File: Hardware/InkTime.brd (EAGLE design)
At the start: 46 x 35 mm, 105 parts, among them IC1 BQ25180YBGR, IC2 DRV2605YZFR, IC3 BMA423, IC9 RT6160AWSC, J1 503480-2400, J2 TC2030-IDC, J4 KH-TYPE-C-16P, Q1 20V/4.2A/52mΩ/1.4W, Q3 SI1308EDL-T1-GE3, U1 NRF52840_QF, U3 MAX17048G+T10, X1 32MHz, X2 32.768kHz

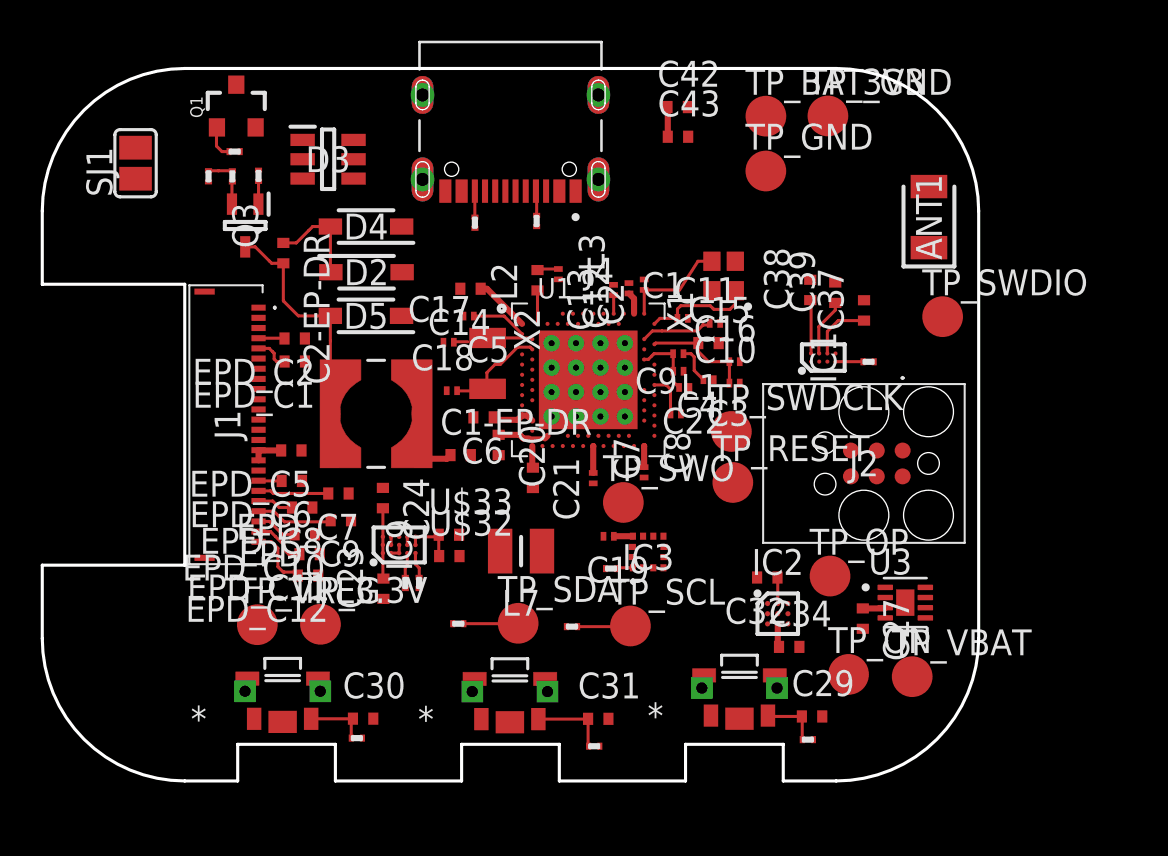
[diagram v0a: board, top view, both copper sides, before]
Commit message: Add files via upload
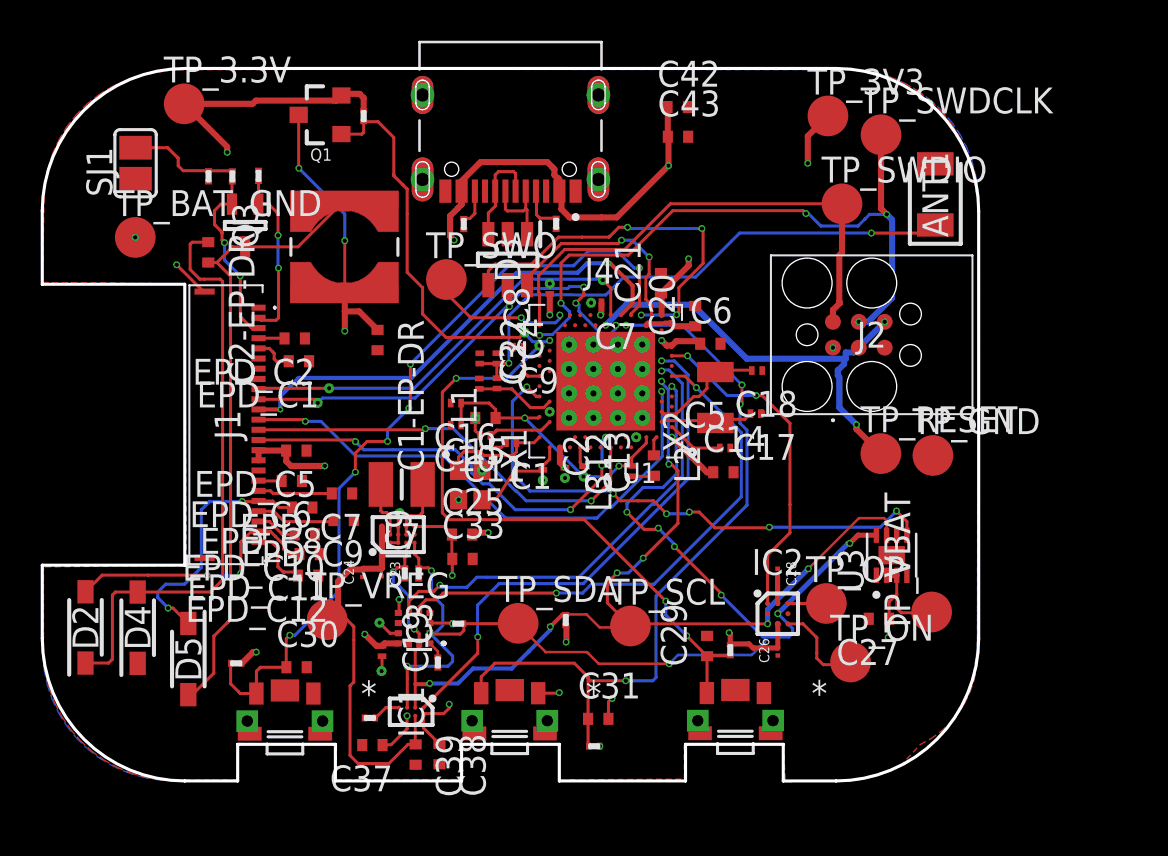
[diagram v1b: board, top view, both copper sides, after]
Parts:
- removed C32: 1uF, InkTime_v5:NORDIC_NRF_3_RESC0402_L
- removed C34: 0.1uF, InkTime_v5:NORDIC_NRF_3_RESC0402_L
- removed U$32, U$33: (no value), InkTime_v5:NORDIC_NRF_3_RESC0402_L
- added C25, C33: (no value), InkTime_v5:NORDIC_NRF_3_RESC0402_L
- added C26, C28: 0.1uF, InkTime_v5:GRM011R60J152KE01L_2_CAPC0201X13N
- C23, C24: device InkTime_v5:NORDIC_NRF_3_RESC0402_L -> InkTime_v5:GRM011R60J152KE01L_2_CAPC0201X13N
- moved C37 32.2 mm to (-6.78, -15.7), turned to 180 degrees
- moved TP_BAT_GND 31.5 mm to (-18.4, 9.20)
- moved C39 30.7 mm to (-4.66, -16.2), turned to 270 degrees
- moved R9 30.1 mm to (-6.91, -14.4), turned to 90 degrees
- moved C38 29.2 mm to (-3.49, -16.2), turned to 270 degrees
- moved IC1 26.7 mm to (-4.88, -14.1), turned to 270 degrees
- moved TP_3.3V 26.4 mm to (-16.0, 15.8)
- moved D4 22.7 mm to (-18.3, -9.97), turned to 90 degrees
- moved D2 22.2 mm to (-20.9, -9.96), turned to 90 degrees
- moved D5 19.0 mm to (-15.8, -11.5), turned to 270 degrees
- moved TP_SWDCLK 16.3 mm to (18.2, 14.2)
- moved TP_GND 16.2 mm to (20.8, -1.51)
- moved X1 16.1 mm to (-1.97, -2.96), turned to 270 degrees
- moved C17 15.5 mm to (12.0, 0.54), turned to 180 degrees
- moved C14 15.3 mm to (10.5, -2.34), turned to 0 degrees
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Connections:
- net 3V3: now also C25.1, C26.2, C33.1; no longer C34.1, U$32.1, U$33.1
- net GND: now also C23.2, C25.2, C26.1, C28.1, C33.2; no longer C23.1, C32.2, C34.2, U$32.2, U$33.2
- net N$63: now also C28.2; no longer C32.1
- net VREG: now also C23.1; no longer C23.2
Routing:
- net 3V3: track 13.1 -> 99.8 mm, vias 0 -> 16
- net VBUS: track 5.18 -> 59.5 mm, vias 0 -> 5
- net SDA: track 3.95 -> 56.9 mm, vias 0 -> 11
- net SCL: track 3.85 -> 52.4 mm, vias 0 -> 10
- net P0.13: track 3.04 -> 39.8 mm, vias 0 -> 6
- net P0.14: track 3.80 -> 36.8 mm, vias 0 -> 4
- net VBAT: track 4.22 -> 37.2 mm, vias 0 -> 2
- net SWDCLK: track 0.00 -> 32.7 mm, vias 0 -> 5
- net P1.02: track 2.83 -> 30.9 mm, vias 0 -> 4
- net ALERT: track 0.00 -> 27.1 mm, vias 0 -> 6
- net EPD_CS: track 0.00 -> 26.3 mm, vias 0 -> 2
- net IMU_INT1: track 0.00 -> 26.1 mm, vias 0 -> 2
- net PMIC_INT: track 0.00 -> 25.8 mm, vias 0 -> 2
- net SWDIO: track 0.00 -> 24.8 mm
- net N$31: track 4.90 -> 28.9 mm
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- added copper zone on layer 15, net 3V3
- added copper zone on layer 1, net GND
- added copper zone on layer 16, net GND
- added copper zone on layer 2, net GND
